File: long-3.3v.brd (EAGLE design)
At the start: 50 x 50 mm, 44 parts, among them J1 CON_HEADER_1X06-SMD-RIGHT-ANG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, Q1 BSS84, U2 MCP73831, U3 MCP9808T-E/MC, U4 ADXL375BCCZ, X1 Micro USB, X2 CRYSTAL, X3 CRYSTALS-NOGND-IQXC-25

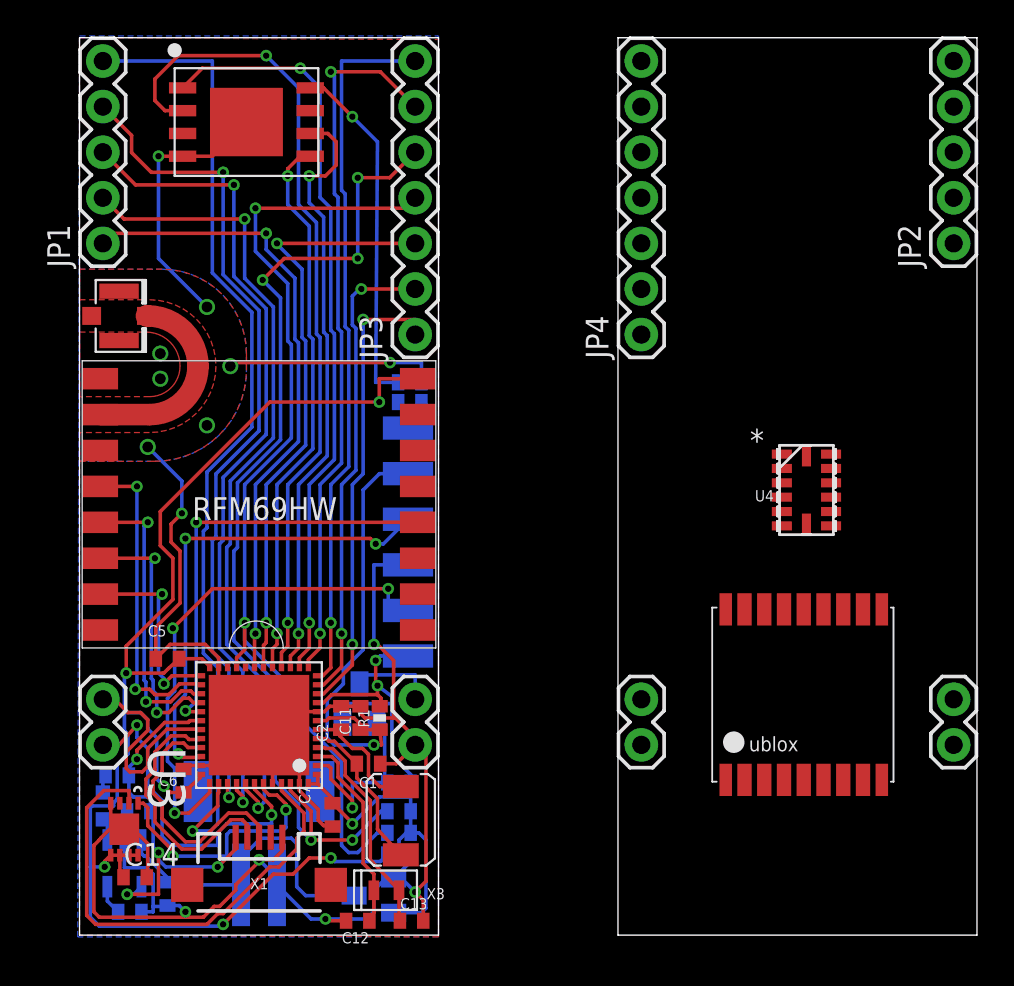
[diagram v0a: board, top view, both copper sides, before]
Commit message: Changed layout, routed board
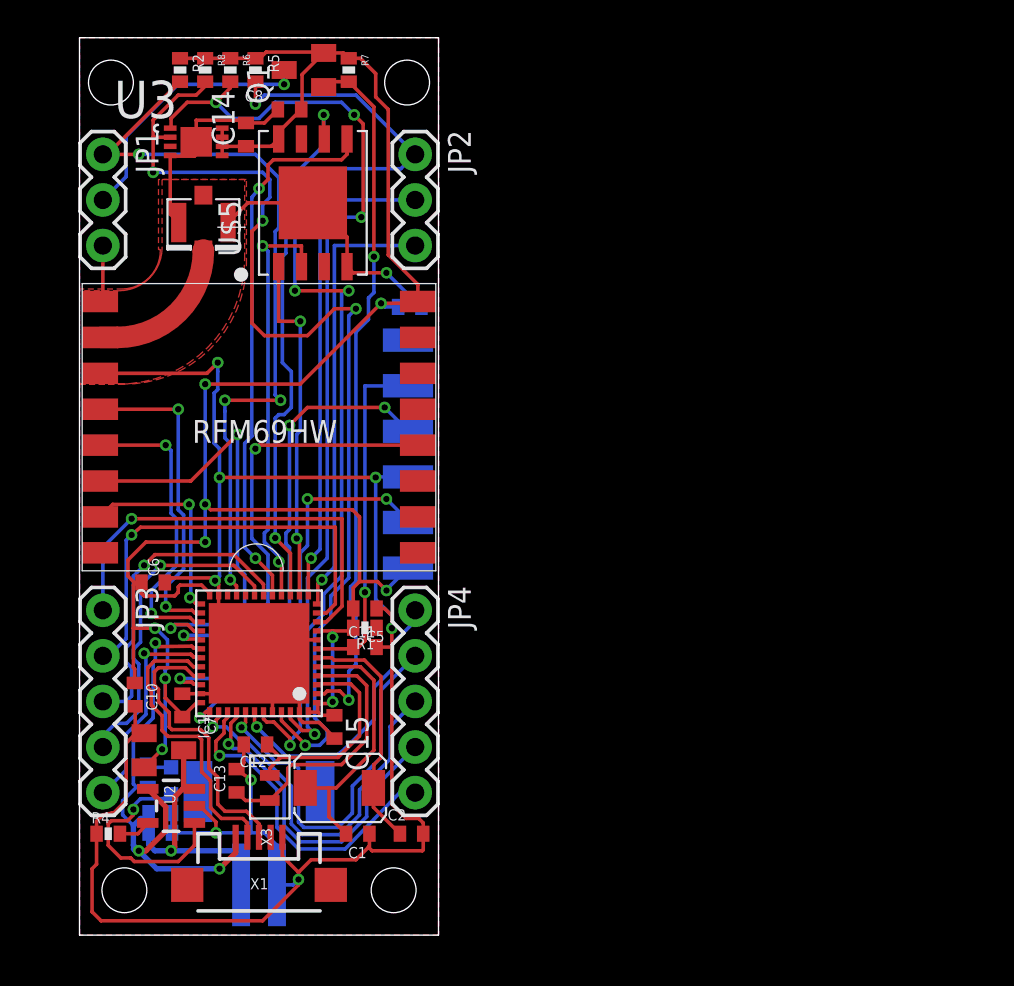
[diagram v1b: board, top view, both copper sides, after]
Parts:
- removed JP14, JP15, JP16, JP17: M02PTH, SparkFun-Connectors:1X02
- removed U$2: UBLOX_MAX, Ava:UBLOX_MAX
- removed U4: ADXL375BCCZ, adxl375bccz:LGA_CC-14-1
- added C15: 100nF, rcl:C0402
- added R6, R8: 3k3, SparkFun:0402-RES
- JP1, JP2: device SparkFun:1X05 -> SparkFun:1X03
- JP3, JP4: device SparkFun:1X07 -> SparkFun:1X05
- moved R2 44.2 mm to (5.60, 48.2), flipped to the top, turned to 270 degrees
- moved R5 42.1 mm to (9.80, 48.2), flipped to the top, turned to 270 degrees
- moved C14 41.8 mm to (9.28, 44.6), turned to 90 degrees
- moved R7 39.8 mm to (15.0, 48.2), flipped to the top, turned to 270 degrees
- moved U3 38.5 mm to (6.50, 44.2), turned to 0 degrees
- moved Q1 35.4 mm to (12.5, 48.2), flipped to the top, turned to 90 degrees
- moved JP2 30.4 mm to (18.7, 43.5), turned to 270 degrees
- moved JP3 23.2 mm to (1.30, 18.1), turned to 270 degrees
- moved JP4 19.9 mm to (18.7, 18.1), turned to 270 degrees
- moved C8 17.6 mm to (11.7, 46.0), flipped to the top
- moved C10 17.2 mm to (3.08, 13.4), flipped to the top, turned to 270 degrees
- moved IC1 14.2 mm to (4.70, 10.3), flipped to the top
- moved C13 12.5 mm to (8.75, 8.60), turned to 90 degrees
- moved C12 11.4 mm to (9.80, 10.6)
- moved C5 11.4 mm to (15.9, 18.2), turned to 0 degrees
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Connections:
- removed net UART_RX: JP4.6
- removed net UART_TX: JP4.7
- net EXT_CS: now also JP4.3; no longer JP1.5, JP2.5
- net EXT_MISO: now also JP4.4; no longer JP1.3, JP2.3
- net EXT_MOSI: now also JP4.2; no longer JP1.2, JP2.2
- net EXT_RX: now also JP2.2; no longer JP3.6
- net EXT_SCK: now also JP4.5; no longer JP1.4, JP2.4
- net EXT_TX: now also JP2.3; no longer JP3.7
- net GND: now also C15.2, JP1.3; no longer JP15.2, JP17.2, U$2.10_GND, U$2.12_GND, U$2.1_GND, U4.2, U4.4, U4.5
- net GPIO1: no longer JP4.1
- net GPIO2: no longer JP4.2
- net GPIO3: no longer JP4.3
- net GPIO4: now also JP3.4; no longer JP1.1, JP2.1
- net GPS_RX: now also JP4.1; no longer JP14.2, JP16.2, U$2.3_RXD1
- net GPS_TX: now also JP3.5; no longer JP14.1, JP16.1, U$2.2_TXD1
- net I2C_SCL: now also JP1.1; no longer JP3.4, JP4.4, U4.14
- net I2C_SDA: now also JP2.1; no longer JP3.5, JP4.5, U4.13
- net LOCAL_SCL: now also R8.2
- net LOCAL_SDA: now also R6.2
- net VCC: now also C15.1, R6.1, R8.1; no longer U$2.14_VCC_RF, U$2.6_V_BCKP, U$2.7_VCC_IO, U$2.8_VCC, U$2.9_V_RESET, U4.1, U4.6
- net VCC_SW: now also JP1.2; no longer JP15.1, JP17.1
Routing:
- net LOCAL_SDA: track 14.8 -> 54.5 mm, vias 2 -> 4
- net EXT_CS: track 55.8 -> 20.9 mm
- net LOCAL_SCL: track 27.4 -> 58.5 mm, vias 0 -> 4
- net EXT_SW: track 10.7 -> 39.4 mm, vias 1 -> 2
- net EXT_SCK: track 46.7 -> 18.4 mm, vias 2 -> 1
- net EXT_MISO: track 46.0 -> 18.7 mm, vias 2 -> 1
- net EXT_MOSI: track 45.6 -> 21.7 mm, vias 2 -> 1
- net FLASH_MISO: track 45.9 -> 23.3 mm
- net FLASH_CS: track 41.9 -> 19.6 mm
- net GND: track 148.2 -> 167.8 mm, vias 14 -> 9
- net VCC: track 137.5 -> 118.1 mm
- net GPIO4: track 35.2 -> 18.3 mm, vias 2 -> 1
- net GPIO3: track 32.9 -> 17.8 mm, vias 2 -> 1
- net EXT_TX: track 39.4 -> 24.9 mm
- net EXT_RX: track 39.6 -> 27.6 mm, vias 2 -> 1
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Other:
- board size 50 x 50 mm -> 20 x 50 mm
